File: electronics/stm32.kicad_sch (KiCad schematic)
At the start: 33 parts, among them J1 USB_B_Micro, J2 Conn_ARM_JTAG_SWD_10, SW1 PTS645SK50SMTR92LFS, U1 USBLC6-2SC6, U2 STM32G431CBUx, Y1 Crystal_GND24

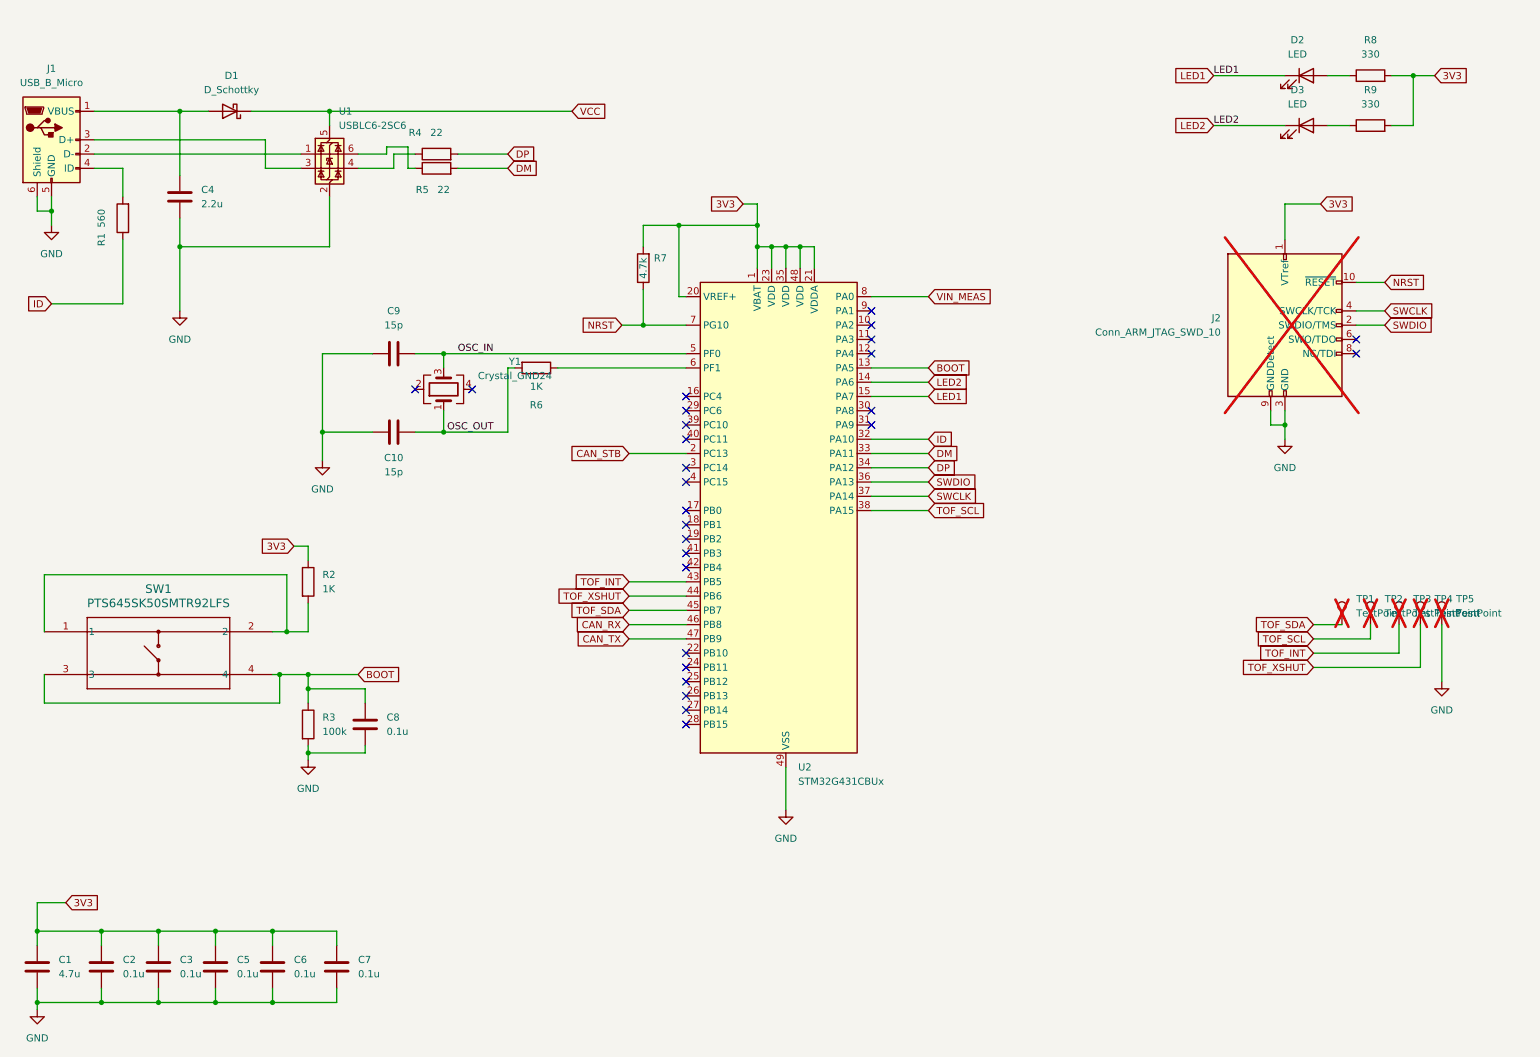
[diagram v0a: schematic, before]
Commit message: Major refactor to rev B
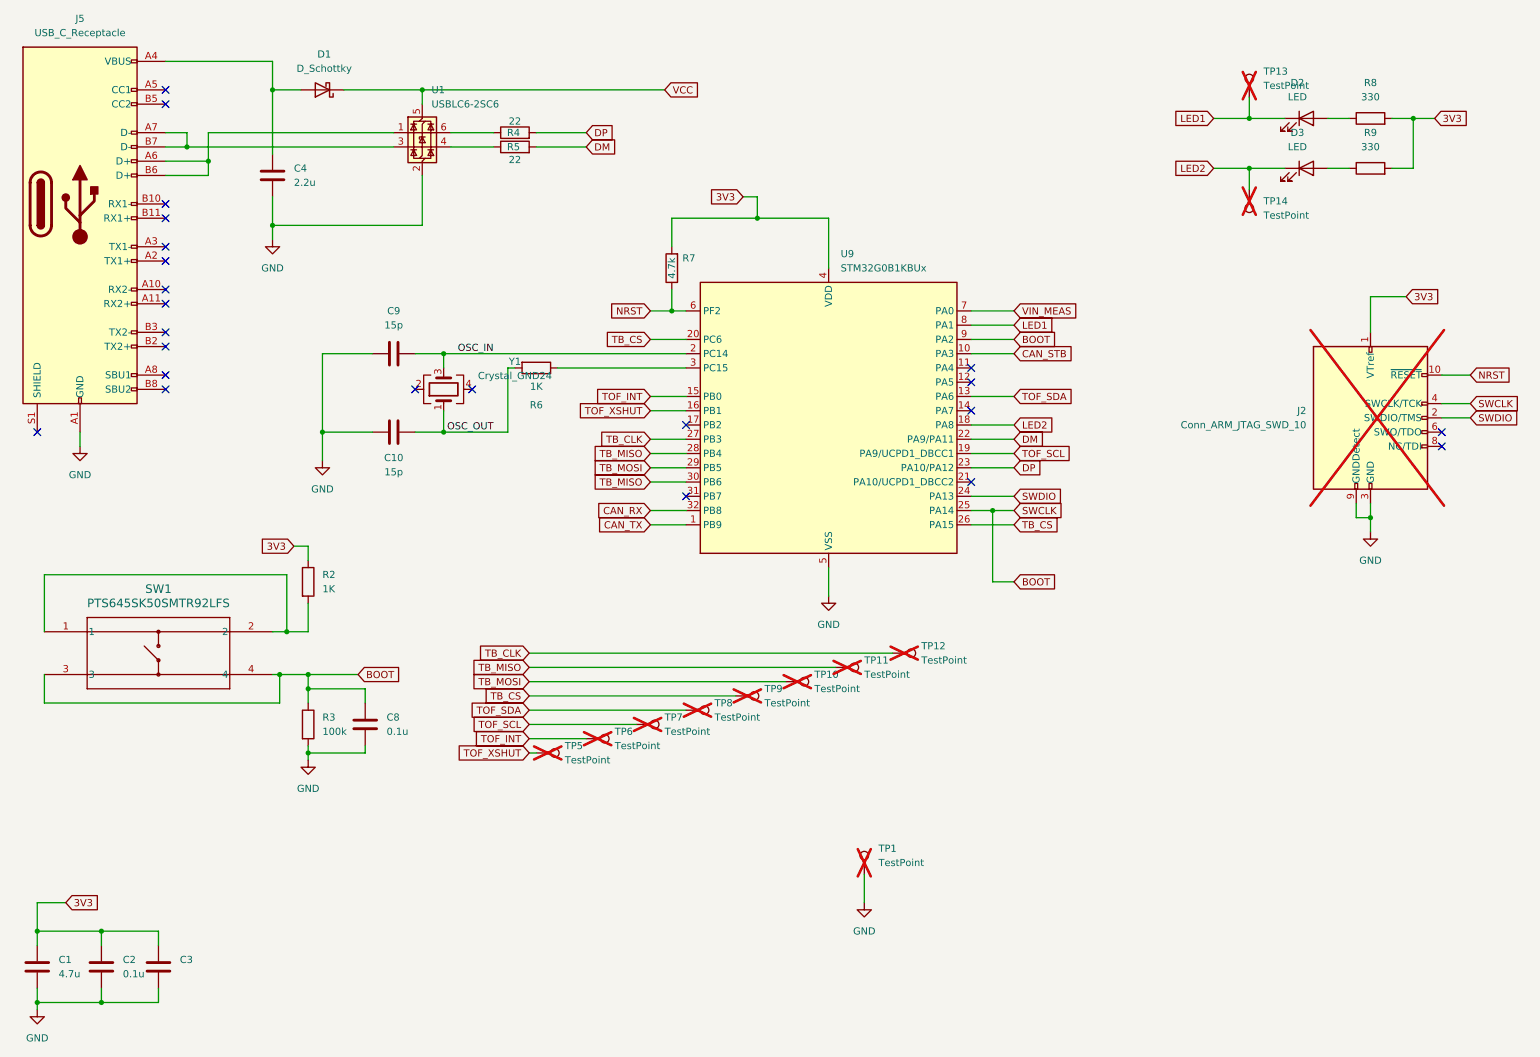
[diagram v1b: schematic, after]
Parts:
- removed C5, C6, C7: 0.1u, Capacitor_SMD:C_0402_1005Metric, symbol Device:C
- removed J1: USB_B_Micro, Connector_USB:USB_Micro-B_Amphenol_10118193-0001LF_Horizontal, symbol Connector:USB_B_Micro
- removed R1: 560, Resistor_SMD:R_0402_1005Metric, symbol Device:R
- removed TP2, TP3, TP4: TestPoint, TestPoint:TestPoint_Pad_D1.0mm, symbol Connector:TestPoint
- removed U2: STM32G431CBUx, Package_DFN_QFN:QFN-48-1EP_7x7mm_P0.5mm_EP5.6x5.6mm, symbol MCU_ST_STM32G4:STM32G431CBUx
- added J5: USB_C_Receptacle, footprints:CONN_105450-0101_MOL, symbol Connector:USB_C_Receptacle
- added TP10, TP11, TP12, TP13, TP14, TP6, TP7, TP8, TP9: TestPoint, TestPoint:TestPoint_Pad_D1.0mm, symbol Connector:TestPoint
- added U9: STM32G0B1KBUx, Package_DFN_QFN:QFN-32-1EP_5x5mm_P0.5mm_EP3.45x3.45mm, symbol MCU_ST_STM32G0:STM32G0B1KBUx
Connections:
- net SWCLK is gone; now on net BOOT: J2.4 (SWCLK/TCK)
- net 3V3: now also U9.4 (VDD)
- net BOOT: now also U9.25 (PA14), U9.9 (PA2)
- net CAN_RX: now also U9.32 (PB8)
- net CAN_STB: now also U9.10 (PA3)
- net CAN_TX: now also U9.1 (PB9)
- net DM: now also U9.22 (PA9/PA11)
- net DP: now also U9.23 (PA10/PA12)
- net GND: now also TP1.1, J5.A1 (GND), J5.A12 (GND), J5.B1 (GND), J5.B12 (GND), U9.33 (VSS), U9.5 (VSS); no longer TP5.1
- net LED1: now also TP13.1, U9.8 (PA1)
- net LED2: now also TP14.1, U9.18 (PA8)
- net NRST: now also U9.6 (PF2)
- net OSC_IN: now also U9.2 (PC14)
- net SWDIO: now also U9.24 (PA13)
- net TOF_INT: now also TP6.1, U9.15 (PB0)
- net TOF_SCL: now also TP7.1, U9.19 (PA9/UCPD1_DBCC1)
- net TOF_SDA: now also TP8.1, U9.13 (PA6); no longer TP1.1
- net TOF_XSHUT: now also TP5.1, U9.16 (PB1)
- net VIN_MEAS: now also U9.7 (PA0)
- net at R5.1: now also U1.4 (I/O2); no longer U1.6 (I/O1)
- net at C4.2, D1.2 (A): now also J5.A4 (VBUS), J5.A9 (VBUS), J5.B4 (VBUS), J5.B9 (VBUS)
- net at R6.1: now also U9.3 (PC15)
- net at U1.1 (I/O1): now also J5.A6 (D+), J5.B6 (D+)
- net at U1.3 (I/O2): now also J5.A7 (D-), J5.B7 (D-)
- net at R4.1: now also U1.6 (I/O1); no longer U1.4 (I/O2)
- new net TB_CLK: TP12.1, U9.27 (PB3)
- new net TB_CS: TP9.1, U9.20 (PC6), U9.26 (PA15)
- new net TB_MISO: TP11.1, U9.28 (PB4), U9.30 (PB6)
- new net TB_MOSI: TP10.1, U9.29 (PB5)
- no-connect marks 27 -> 23
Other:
- moved on the sheet: C4, D1, D2, D3, J2, R4, R5, R7, R8, R9, U1
